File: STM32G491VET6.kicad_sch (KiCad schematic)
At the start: 36 parts, among them J2 TC2030, J3 CAN_CONNECTOR, U2 TYPE-C 16PLT-H10.0, U3 STM32G431CBT6, U9 C31086109, X1 X50328MSB2GI, Y1 SSPT7F-7PF20-R

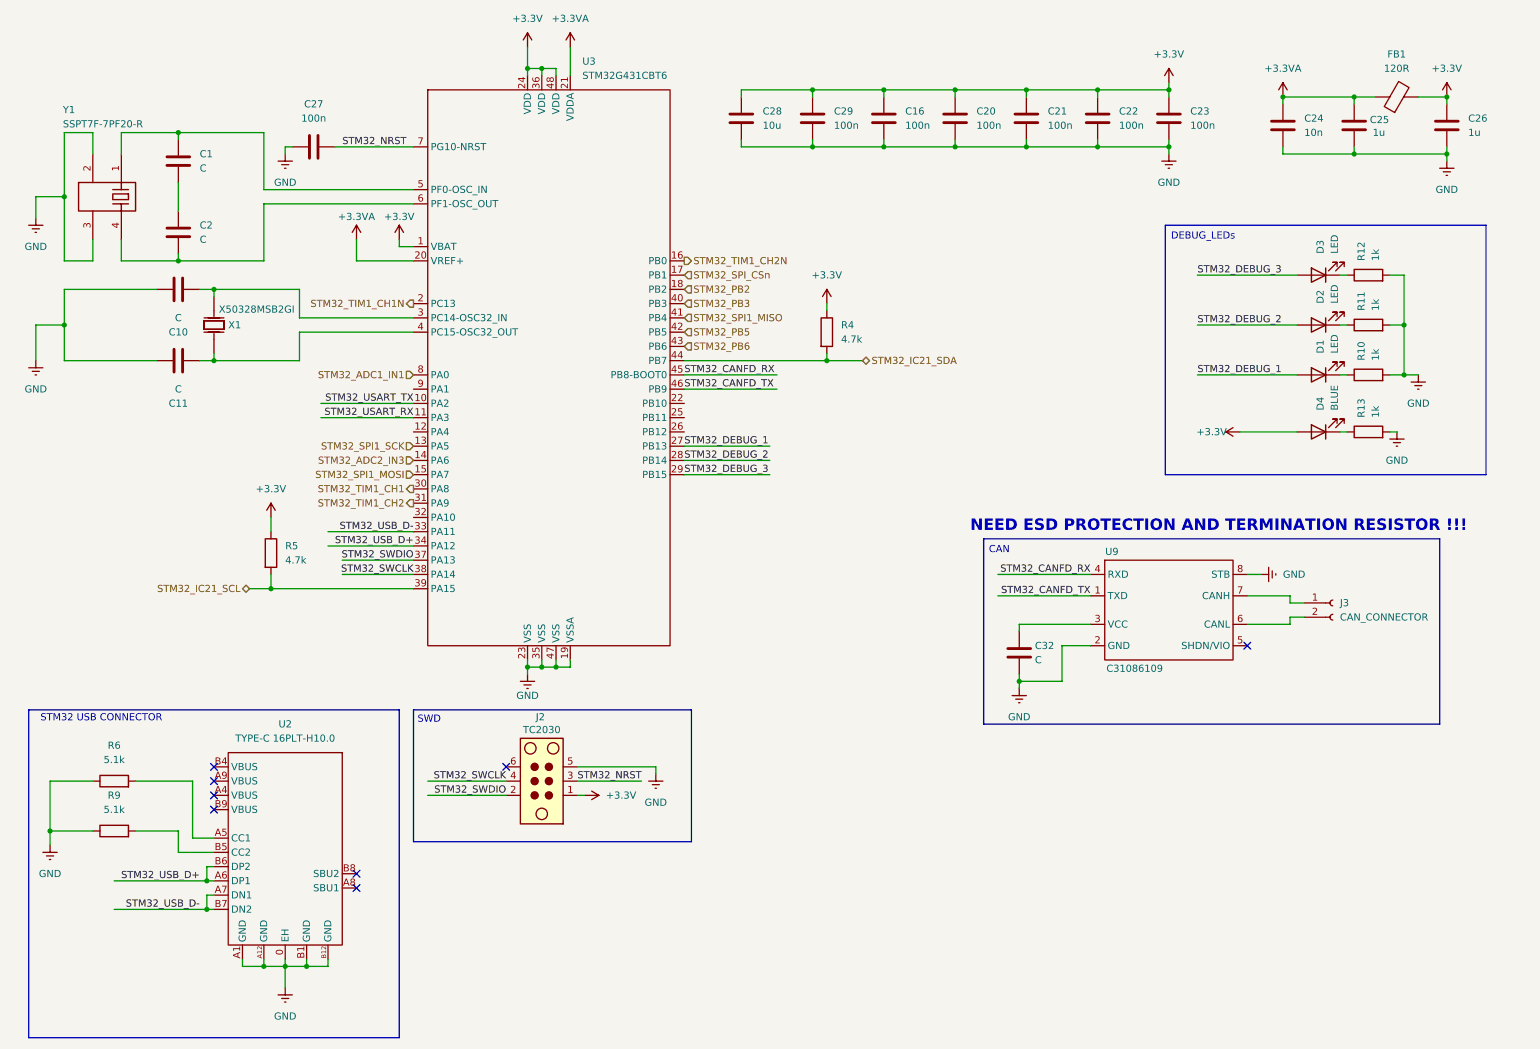
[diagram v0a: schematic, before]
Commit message: change components
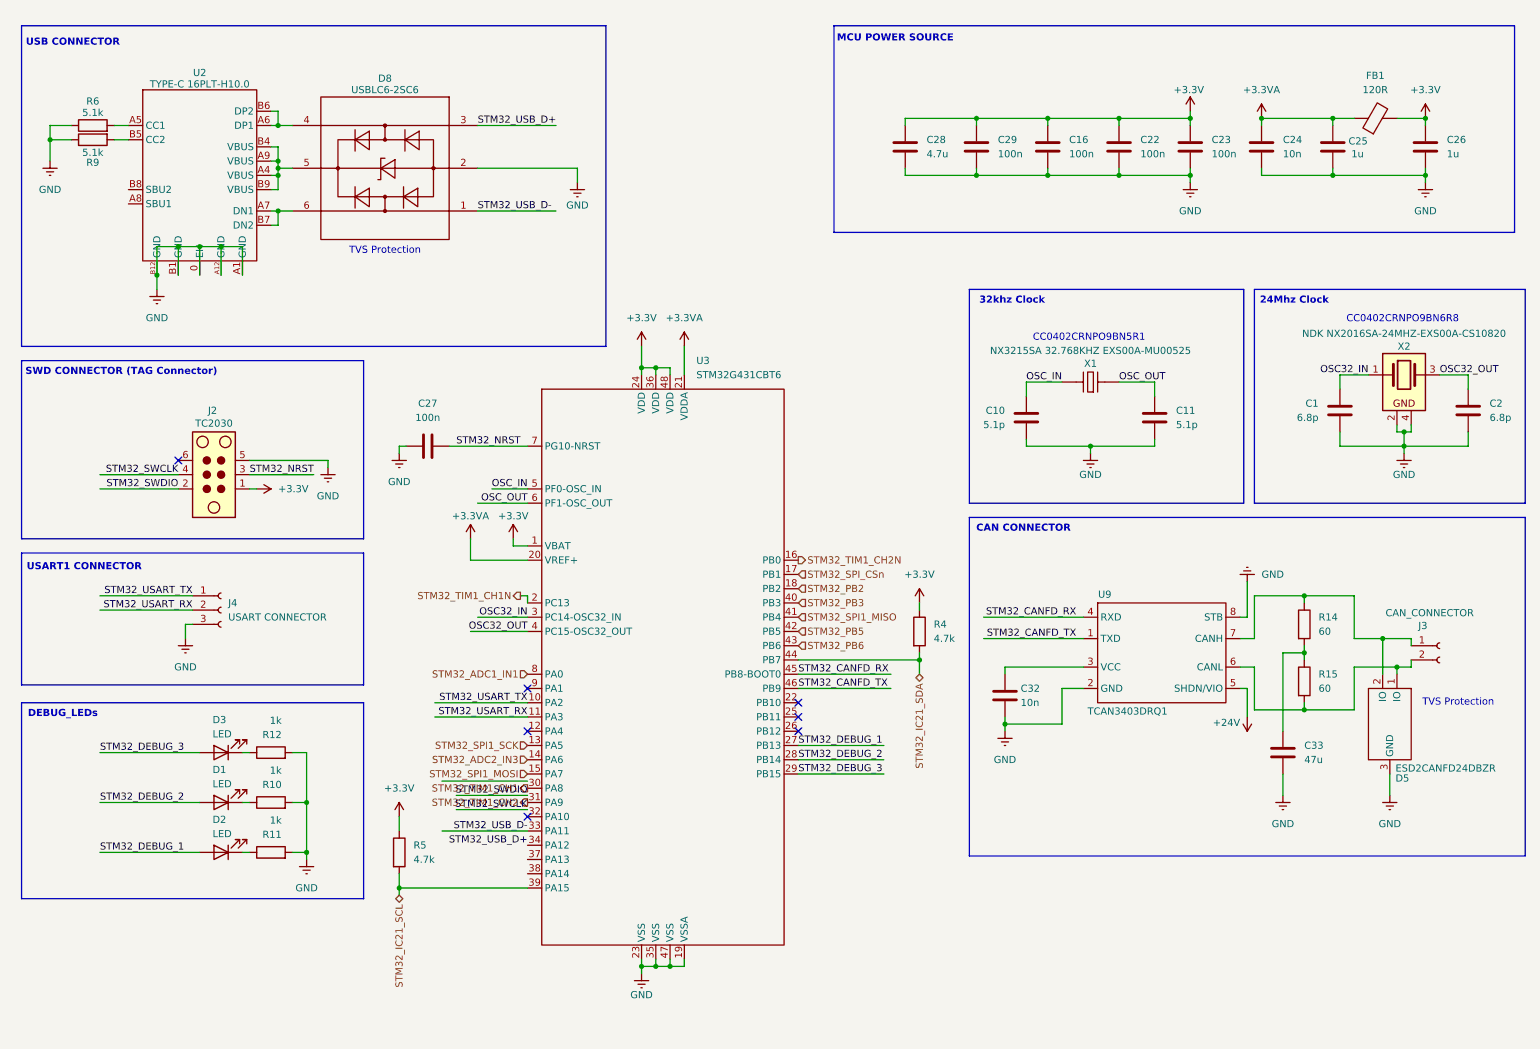
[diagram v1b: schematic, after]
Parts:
- removed C20, C21: 100n, symbol Device:C
- removed D4: BLUE, symbol Device:LED
- removed R13: 1k, symbol Device:R
- removed X1: X50328MSB2GI, EasyEDA_Lib:CRYSTAL-SMD_L5.0-W3.2, symbol EasyEDA_Lib:X50328MSB2GI
- removed Y1: SSPT7F-7PF20-R, EasyEDA_Lib:MC-146_4P-L6.7-W1.5-P0.85-BL, symbol EasyEDA_Lib:32.768kHz
- added C33: 47u, Capacitor_SMD:C_0402_1005Metric, symbol Device:C
- added D5: ESD2CANFD24DBZR, EasyEDA_Lib:SOT-23-3_L2.9-W1.3-P1.90-LS2.4-BL-2, symbol EasyEDA_Lib:ESD2CANFD24DBZR
- added D8: USBLC6-2SC6, EasyEDA_Lib:SOT-23-6_L2.9-W1.6-P0.95-LS2.8-BL, symbol EasyEDA_Lib:USBLC6-2SC6
- added J4: USART CONNECTOR, symbol Connector:Conn_01x03_Socket
- added R14, R15: 60, PCM_Resistor_SMD_AKL:R_0402_1005Metric, symbol Device:R
- added X1: NX3215SA 32.768KHZ EXS00A-MU00525, EasyEDA_Lib:CRYSTAL-SMD_L3.2-W1.5, symbol EasyEDA_Lib:NX3215SA 32.768KHZ EXS00A-MU00525
- added X2: NDK NX2016SA-24MHZ-EXS00A-CS10820, PCM_Crystal_AKL:Crystal_SMD_2016-4Pin_2.0x1.6mm, symbol PCM_Crystal_AKL:SMD2016-4
- C1, C2: value C -> 6.8p; footprint (none) -> Capacitor_SMD:C_0402_1005Metric
- C10, C11: value C -> 5.1p; footprint (none) -> PCM_JLCPCB:C_0603
- C16, C22, C23, C24, C25, C26, C27, C29: footprint (none) -> Capacitor_SMD:C_0402_1005Metric
- C28: value 10u -> 4.7u; footprint (none) -> Capacitor_SMD:C_0402_1005Metric
- C32: value C -> 10n; footprint (none) -> Capacitor_SMD:C_0402_1005Metric
- R10, R11, R12, R4, R5, R6, R9: footprint (none) -> PCM_Resistor_SMD_AKL:R_0402_1005Metric
- U9: value C31086109 -> TCAN3403DRQ1
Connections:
- net GND: now also C1.2, C2.2, C33.2, D5.3 (GND), D8.2, J4.3 (Pin_3), X2.2, X2.4
- net STM32_DEBUG_1: now also D2.2 (A); no longer D1.2 (A)
- net STM32_DEBUG_2: now also D1.2 (A); no longer D2.2 (A)
- net STM32_SWCLK: no longer U3.38 (PA14)
- net STM32_SWDIO: no longer U3.37 (PA13)
- net STM32_USART_RX: now also J4.2 (Pin_2)
- net STM32_USART_TX: now also J4.1 (Pin_1)
- net STM32_USB_D+: now also D8.3; no longer U2.A6 (DP1), U2.B6 (DP2)
- net STM32_USB_D-: now also D8.1; no longer U2.A7 (DN1), U2.B7 (DN2)
- net OSC32_IN: now reaches C1.1
- net OSC32_IN: now also U3.3 (PC14-OSC32_IN), X2.1; no longer U3.5 (PF0-OSC_IN)
- net OSC32_OUT: now reaches C2.1
- net OSC32_OUT: now also U3.4 (PC15-OSC32_OUT), X2.3; no longer C1.2
- net OSC_OUT: now reaches C11.1
- net OSC_OUT: now also U3.6 (PF1-OSC_OUT), X1.1; no longer U3.4 (PC15-OSC32_OUT)
- net at J3.1 (Pin_1), U9.7 (CANH): now also D5.2 (IO), R14.1
- net at J3.2 (Pin_2), U9.6 (CANL): now also D5.1 (IO), R15.2
- net at U2.A4 (VBUS): now also U2.A9 (VBUS), U2.B4 (VBUS), U2.B9 (VBUS), D8.5
- net OSC_IN: now reaches C10.1
- net OSC_IN: now also U3.5 (PF0-OSC_IN), X1.2; no longer U3.3 (PC14-OSC32_IN)
- net +24V: now reaches U9.5 (SHDN/VIO)
- new net: C33.1, R14.2, R15.1
- new net: D8.4, U2.A6 (DP1), U2.B6 (DP2)
- new net: D8.6, U2.A7 (DN1), U2.B7 (DN2)
- no-connect marks 8 -> 7
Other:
- note added: "24Mhz Clock"
- note added: "32khz Clock"
- note added: "CAN CONNECTOR"
- note added: "CC0402CRNPO9BN5R1"
- note added: "CC0402CRNPO9BN6R8"
- note added: "MCU POWER SOURCE"
- note added: "SWD CONNECTOR (TAG Connector)"
- note added: "TVS Protection"
- note added: "USART1 CONNECTOR"
- note added: "USB CONNECTOR"
- note removed: "CAN"
- note removed: "NEED ESD PROTECTION AND TERMINATION RESISTOR !!!"
- note removed: "STM32 USB CONNECTOR"
- note removed: "SWD"
- moved on the sheet: C16, C22, C23, C24, C25, C26, C27, C28, C29, C32, D3, FB1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
